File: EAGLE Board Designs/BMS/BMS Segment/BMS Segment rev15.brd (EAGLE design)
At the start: 240.3 x 108 mm, 239 parts, among them J0 CONNECTOR-1, J1 CONNECTOR-1, J10 CONNECTOR-1, J11 CONNECTOR-1, J12 CONNECTOR-1, J13 CONNECTOR-1, J14 CONNECTOR-1, J15 CONNECTOR-1, J16 CONNECTOR-1, J17 CONNECTOR-1, J18 CONNECTOR-1, J2 CONNECTOR-1, J3 CONNECTOR-1, J4 CONNECTOR-1, J5 CONNECTOR-1, J6 CONNECTOR-1, J7 CONNECTOR-1, J8 CONNECTOR-1, J9 CONNECTOR-1, T1 TRANSFORMER, U1 LTC6813

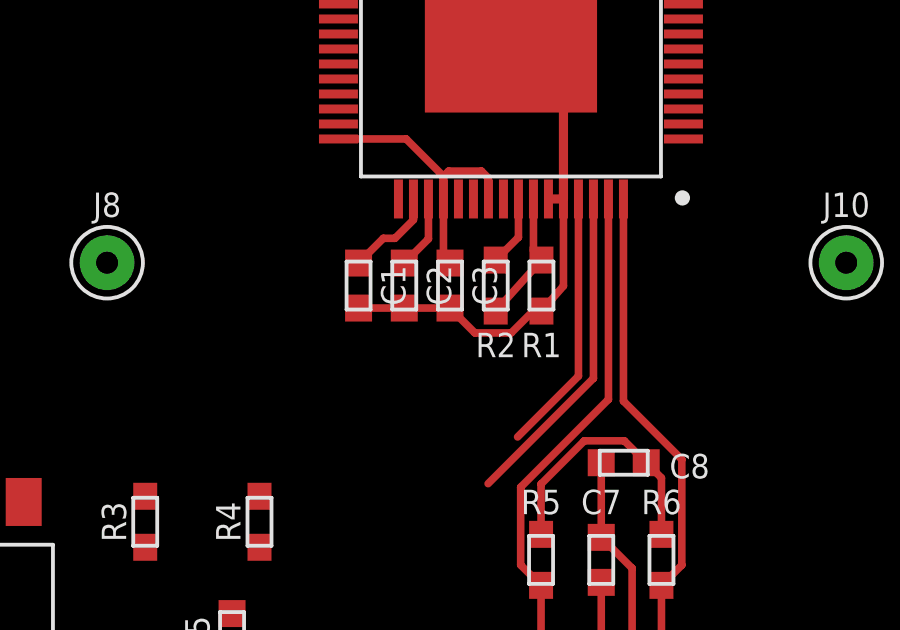
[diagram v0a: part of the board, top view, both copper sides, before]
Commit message: Last commit? :(
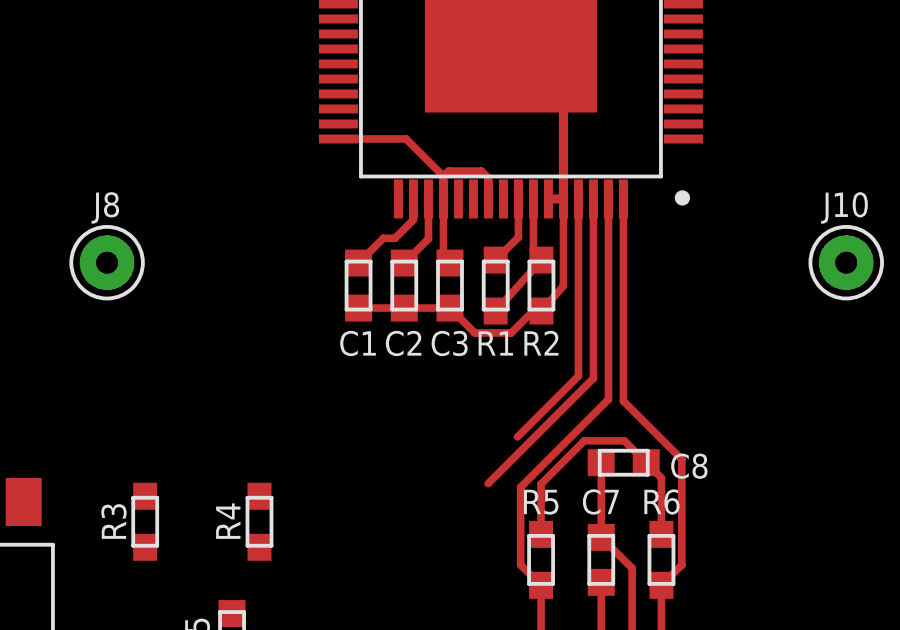
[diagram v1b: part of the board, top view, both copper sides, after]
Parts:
- moved R1 1.52 mm to (120.9, -74.7)
- moved R2 1.52 mm to (122.4, -74.7)
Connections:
- net IBIAS: now also R1.2; no longer R2.2
- net ICMP: now also R1.1, R2.2; no longer R1.2, R2.1
- net V-: now also R2.1; no longer R1.1
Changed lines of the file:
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@@
 <attribute name="MOPN" value="603-CC603KRX7R6BB105" x="116.332" y="-74.676" size="1.778" layer="27" rot="R270" display="off"/>
 <attribute name="MPN" value="CC0603KRX7R6BB105" x="116.332" y="-74.676" size="1.778" layer="27" rot="R270" display="off"/>
-<attribute name="NAME" x="117.082" y="-74.676" size="0.8128" layer="25" font="vector" rot="R270" align="bottom-center"/>
+<attribute name="NAME" x="116.332" y="-76.2" size="0.8128" layer="25" font="vector" align="top-center"/>
 <attribute name="TOLERANCE" value="10%" x="116.332" y="-74.676" size="1.778" layer="27" rot="R270" display="off"/>
 <attribute name="VOLTAGE" value="10V" x="116.332" y="-74.676" size="1.778" layer="27" rot="R270" display="off"/>
@@
 <attribute name="MOPN" value="603-CC603KRX7R6BB105" x="117.856" y="-74.676" size="1.778" layer="27" rot="R270" display="off"/>
 <attribute name="MPN" value="CC0603KRX7R6BB105" x="117.856" y="-74.676" size="1.778" layer="27" rot="R270" display="off"/>
-<attribute name="NAME" x="118.606" y="-74.676" size="0.8128" layer="25" font="vector" rot="R270" align="bottom-center"/>
+<attribute name="NAME" x="117.856" y="-76.2" size="0.8128" layer="25" font="vector" align="top-center"/>
 <attribute name="TOLERANCE" value="10%" x="117.856" y="-74.676" size="1.778" layer="27" rot="R270" display="off"/>
 <attribute name="VOLTAGE" value="10V" x="117.856" y="-74.676" size="1.778" layer="27" rot="R270" display="off"/>
@@
 <attribute name="MOPN" value="603-CC603KRX7R6BB105" x="119.38" y="-74.676" size="1.778" layer="27" rot="R270" display="off"/>
 <attribute name="MPN" value="CC0603KRX7R6BB105" x="119.38" y="-74.676" size="1.778" layer="27" rot="R270" display="off"/>
-<attribute name="NAME" x="120.13" y="-74.676" size="0.8128" layer="25" font="vector" rot="R270" align="bottom-center"/>
+<attribute name="NAME" x="119.38" y="-76.2" size="0.8128" layer="25" font="vector" align="top-center"/>
 <attribute name="TOLERANCE" value="10%" x="119.38" y="-74.676" size="1.778" layer="27" rot="R270" display="off"/>
 <attribute name="VOLTAGE" value="10V" x="119.38" y="-74.676" size="1.778" layer="27" rot="R270" display="off"/>
@@
 <attribute name="VOLTAGE" value="100V" x="-615.95" y="-826.77" size="1.778" layer="27" display="off"/>
 </element>
-<element name="R1" library="HyTechDevices" package="0603-RES" value="RESISTOR_0603_1K" x="122.428" y="-74.676" smashed="yes" rot="R90">
+<element name="R2" library="HyTechDevices" package="0603-RES" value="RESISTOR_0603_1K" x="122.428" y="-74.676" smashed="yes" rot="R90">
 <attribute name="DKPN" value="311-1.00KHRCT-ND" x="122.428" y="-74.676" size="1.778" layer="27" rot="R90" display="off"/>
 <attribute name="MANUFACTURER" value="Yageo" x="122.428" y="-74.676" size="1.778" layer="27" rot="R90" display="off"/>
 <attribute name="MOPN" value="603-RC0603FR-071KL" x="122.428" y="-74.676" size="1.778" layer="27" rot="R90" display="off"/>
 <attribute name="MPN" value="RC0603FR-071KL" x="122.428" y="-74.676" size="1.778" layer="27" rot="R90" display="off"/>
-<attribute name="NAME" x="122.428" y="-76.2508" size="0.8128" layer="25" font="vector" align="top-center"/>
+<attribute name="NAME" x="122.428" y="-76.2" size="0.8128" layer="25" font="vector" align="top-center"/>
 <attribute name="POWER" value="0.1W" x="122.428" y="-74.676" size="1.778" layer="27" rot="R90" display="off"/>
 <attribute name="RESISTANCE" value="1k" x="122.428" y="-74.676" size="1.778" layer="27" rot="R90" display="off"/>
@@
 <attribute name="VOLTAGE" value="75V" x="122.428" y="-74.676" size="1.778" layer="27" rot="R90" display="off"/>
 </element>
-<element name="R2" library="HyTechDevices" package="0603-RES" value="RESISTOR_0603_1K" x="120.904" y="-74.676" smashed="yes" rot="R90">
+<element name="R1" library="HyTechDevices" package="0603-RES" value="RESISTOR_0603_1K" x="120.904" y="-74.676" smashed="yes" rot="R90">
 <attribute name="DKPN" value="311-1.00KHRCT-ND" x="120.904" y="-74.676" size="1.778" layer="27" rot="R90" display="off"/>
 <attribute name="MANUFACTURER" value="Yageo" x="120.904" y="-74.676" size="1.778" layer="27" rot="R90" display="off"/>
 <attribute name="MOPN" value="603-RC0603FR-071KL" x="120.904" y="-74.676" size="1.778" layer="27" rot="R90" display="off"/>
 <attribute name="MPN" value="RC0603FR-071KL" x="120.904" y="-74.676" size="1.778" layer="27" rot="R90" display="off"/>
-<attribute name="NAME" x="120.904" y="-76.2508" size="0.8128" layer="25" font="vector" align="top-center"/>
+<attribute name="NAME" x="120.904" y="-76.2" size="0.8128" layer="25" font="vector" align="top-center"/>
 <attribute name="POWER" value="0.1W" x="120.904" y="-74.676" size="1.778" layer="27" rot="R90" display="off"/>
 <attribute name="RESISTANCE" value="1k" x="120.904" y="-74.676" size="1.778" layer="27" rot="R90" display="off"/>
@@
 <signal name="ICMP">
 <contactref element="U1" pad="58"/>
-<contactref element="R1" pad="2"/>
-<contactref element="R2" pad="1"/>
+<contactref element="R2" pad="2"/>
+<contactref element="R1" pad="1"/>
 <wire x1="120.904" y1="-75.526" x2="122.4788" y2="-73.7734" width="0.254" layer="1"/>
 <wire x1="122.4788" y1="-73.7734" x2="122.428" y2="-73.826" width="0.254" layer="1"/>
@@
 <signal name="IBIAS">
 <contactref element="U1" pad="57"/>
-<contactref element="R2" pad="2"/>
+<contactref element="R1" pad="2"/>
 <wire x1="120.904" y1="-73.826" x2="121.662" y2="-73.068" width="0.254" layer="1"/>
 <wire x1="121.662" y1="-73.068" x2="121.662" y2="-71.79" width="0.254" layer="1"/>
@@
 <contactref element="C6" pad="1"/>
 <contactref element="SENSE18.C1" pad="2"/>
-<contactref element="R1" pad="1"/>
+<contactref element="R2" pad="1"/>
 <contactref element="C7" pad="1"/>
 <contactref element="C8" pad="2"/>
